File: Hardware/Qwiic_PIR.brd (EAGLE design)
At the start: 25.4 x 25.4 mm, 48 parts, among them J2 QWIIC, J3 QWIIC, J7 ISP, U1 EKMC4607112k, U4 ATTINY84-ARDUINO

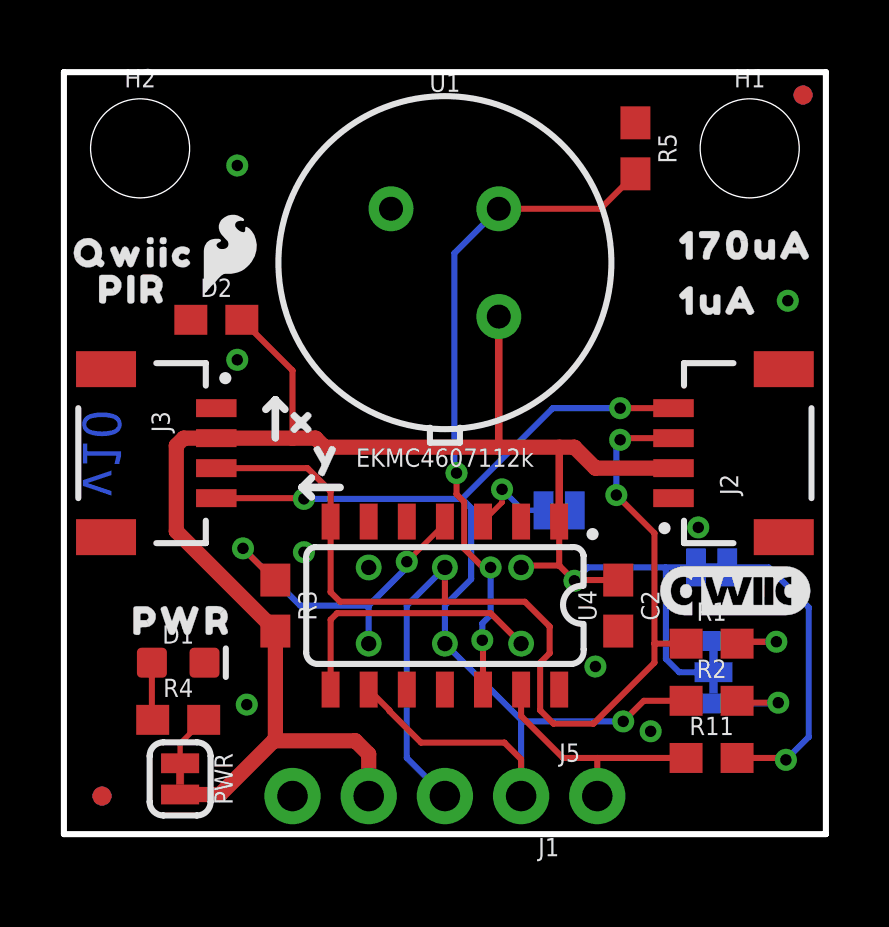
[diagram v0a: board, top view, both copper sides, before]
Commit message: Panelizing
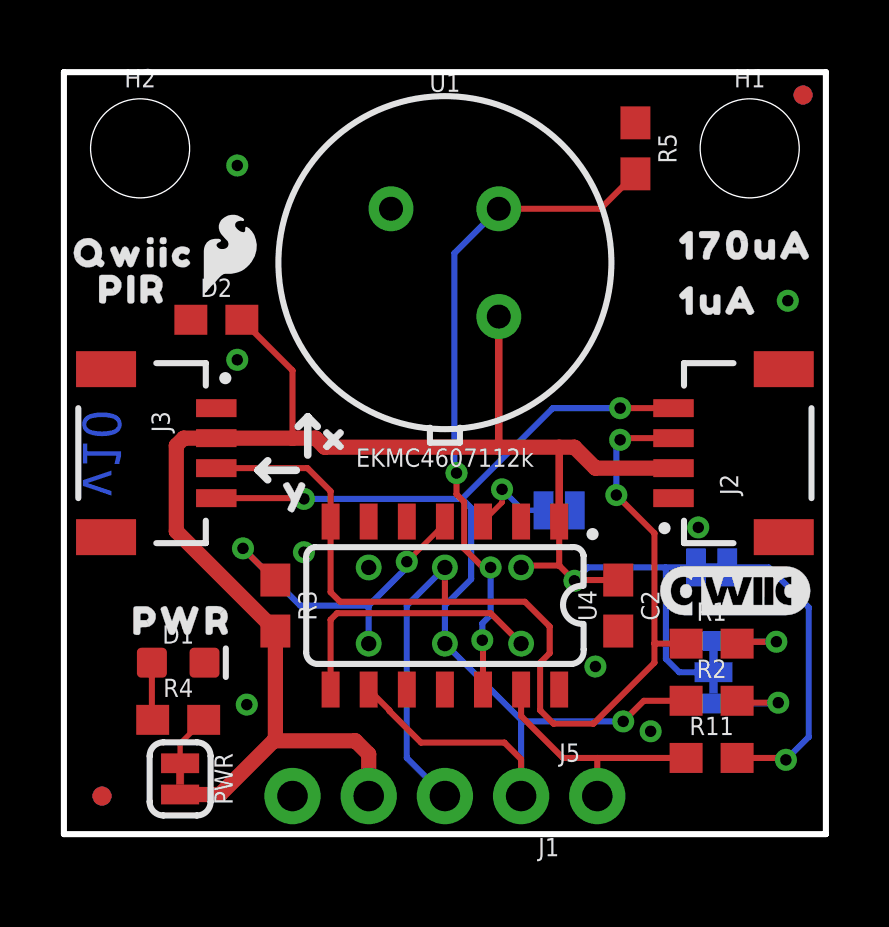
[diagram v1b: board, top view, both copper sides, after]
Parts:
- moved U$16 1.58 mm to (6.60, 11.5)
- moved U$14 1.22 mm to (7.94, 13.3)
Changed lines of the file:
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@@
 <grid distance="0.05" unitdist="inch" unit="inch" style="lines" multiple="1" display="yes" altdistance="0.0025" altunitdist="inch" altunit="inch"/>
 <layers>
-<layer number="1" name="Top" color="4" fill="1" visible="yes" active="yes"/>
-<layer number="16" name="Bottom" color="1" fill="1" visible="yes" active="yes"/>
+<layer number="1" name="Top" color="4" fill="1" visible="no" active="yes"/>
+<layer number="16" name="Bottom" color="1" fill="1" visible="no" active="yes"/>
 <layer number="17" name="Pads" color="2" fill="1" visible="yes" active="yes"/>
-<layer number="18" name="Vias" color="2" fill="1" visible="yes" active="yes"/>
+<layer number="18" name="Vias" color="2" fill="1" visible="no" active="yes"/>
 <layer number="19" name="Unrouted" color="6" fill="1" visible="yes" active="yes"/>
 <layer number="20" name="Dimension" color="24" fill="1" visible="yes" active="yes"/>
@@
 <rectangle x1="19.2405" y1="17.2085" x2="20.32" y2="18.288" layer="29"/>
 <rectangle x1="19.2405" y1="19.05" x2="20.32" y2="20.1295" layer="31"/>
-<wire x1="9.2075" y1="11.557" x2="7.9375" y2="11.557" width="0.254" layer="21"/>
-<wire x1="7.9375" y1="11.557" x2="8.255" y2="11.8745" width="0.254" layer="21"/>
-<wire x1="7.9375" y1="11.557" x2="8.255" y2="11.2395" width="0.254" layer="21"/>
-<wire x1="7.0485" y1="13.208" x2="7.0485" y2="14.478" width="0.254" layer="21"/>
-<wire x1="7.0485" y1="14.478" x2="7.366" y2="14.1605" width="0.254" layer="21"/>
-<wire x1="7.0485" y1="14.478" x2="6.731" y2="14.1605" width="0.254" layer="21"/>
+<wire x1="7.747" y1="12.1285" x2="6.477" y2="12.1285" width="0.254" layer="21"/>
+<wire x1="6.477" y1="12.1285" x2="6.7945" y2="12.446" width="0.254" layer="21"/>
+<wire x1="6.477" y1="12.1285" x2="6.7945" y2="11.811" width="0.254" layer="21"/>
+<wire x1="8.128" y1="12.6365" x2="8.128" y2="13.9065" width="0.254" layer="21"/>
+<wire x1="8.128" y1="13.9065" x2="8.4455" y2="13.589" width="0.254" layer="21"/>
+<wire x1="8.128" y1="13.9065" x2="7.8105" y2="13.589" width="0.254" layer="21"/>
 <dimension x1="2.54" y1="22.86" x2="2.54" y2="25.4" x3="-2.54" y3="24.13" textsize="1.778" layer="47" unit="inch"/>
 <dimension x1="2.54" y1="22.86" x2="0" y2="22.86" x3="1.27" y3="34.29" textsize="1.778" layer="47" unit="inch"/>
@@
 <element name="U$2" library="output" package="170UA0" value="" x="19.812" y="19.6215" smashed="yes"/>
 <element name="U$9" library="output" package="1UA0" value="" x="19.812" y="17.78" smashed="yes"/>
-<element name="U$14" library="output" package="X0" value="" x="6.858" y="13.843" smashed="yes"/>
-<element name="U$16" library="output" package="Y0" value="" x="7.62" y="12.7" smashed="yes"/>
+<element name="U$14" library="output" package="X0" value="" x="7.9375" y="13.2715" smashed="yes"/>
+<element name="U$16" library="output" package="Y0" value="" x="6.604" y="11.4935" smashed="yes"/>
 <element name="U$17" library="output" package="QWIIC0" value="" x="-0.381" y="19.3675" smashed="yes"/>
 <element name="U$18" library="output" package="QWIIC0" value="" x="16.764" y="19.05" smashed="yes" rot="MR0"/>
